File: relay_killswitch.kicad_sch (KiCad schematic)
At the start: 4 parts, among them Q1 BSN20, Q4 Q_PMOS_DGS

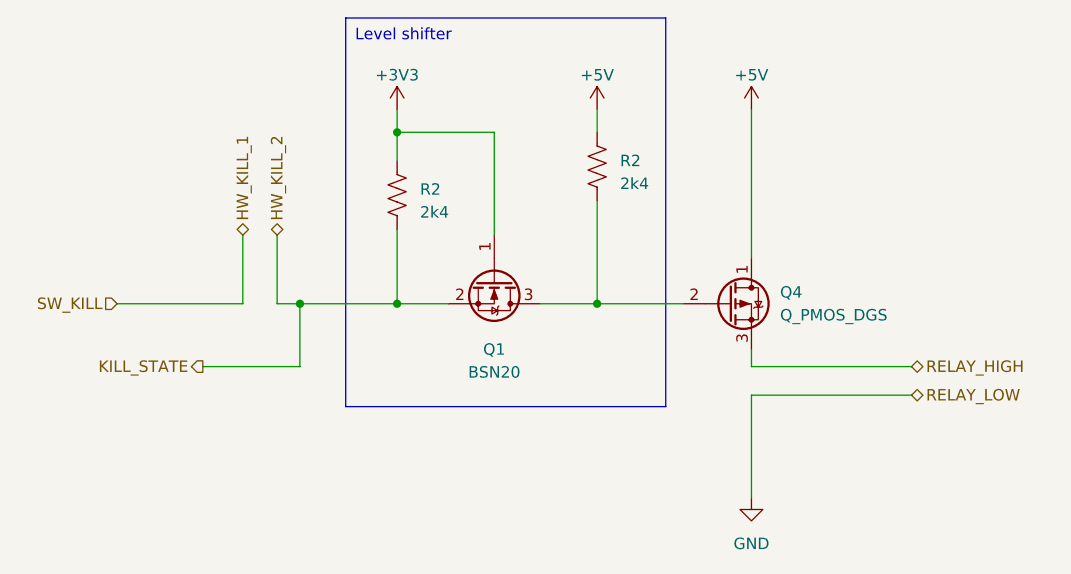
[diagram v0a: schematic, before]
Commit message: Start laying out main board
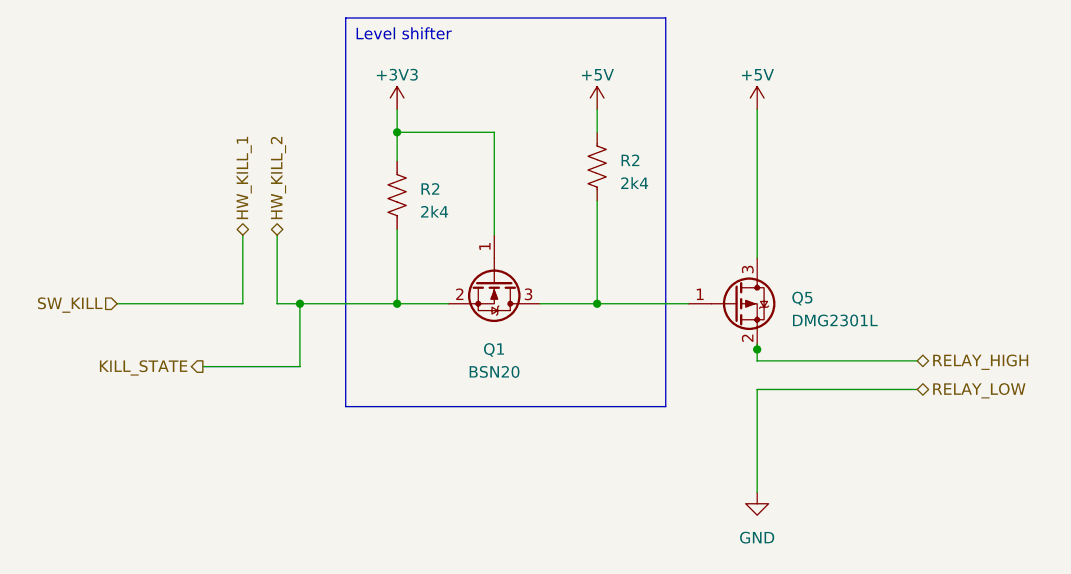
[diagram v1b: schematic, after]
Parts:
- removed Q4: Q_PMOS_DGS, symbol Device:Q_PMOS_DGS
- added Q5: DMG2301L, Package_TO_SOT_SMD:SOT-23, symbol Transistor_FET:DMG2301L
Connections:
- net +5V: now also Q5.3 (D)
- net RELAY_HIGH: now also Q5.2 (S)
- net at Q1.3 (D), R2.2: now also Q5.1 (G)
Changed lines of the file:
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@@
   (junction (at 34.29 49.53) (diameter 0) (color 0 0 0 0)
   )
+  (junction (at 85.09 54.61) (diameter 0) (color 0 0 0 0)
+  )
   (junction (at 45.085 49.53) (diameter 0) (color 0 0 0 0)
   )
@@
   (junction (at 45.085 30.48) (diameter 0) (color 0 0 0 0)
   )
-  (wire (pts (xy 84.455 27.94) (xy 84.455 44.45))
+  (wire (pts (xy 85.09 27.94) (xy 85.09 44.45))
     (stroke (width 0) (type default))
   )
@@
     (stroke (width 0) (type default))
   )
+  (wire (pts (xy 85.09 54.61) (xy 85.09 53.975))
+    (stroke (width 0) (type default))
+  )
   (wire (pts (xy 31.75 49.53) (xy 34.29 49.53))
     (stroke (width 0) (type default))
@@
     (stroke (width 0) (type default))
   )
-  (wire (pts (xy 84.455 56.515) (xy 102.235 56.515))
+  (wire (pts (xy 85.09 55.88) (xy 102.87 55.88))
     (stroke (width 0) (type default))
   )
@@
     (stroke (width 0) (type default))
   )
-  (wire (pts (xy 84.455 59.69) (xy 84.455 71.12))
-    (stroke (width 0) (type default))
-  )
-  (wire (pts (xy 67.31 49.53) (xy 76.835 49.53))
-    (stroke (width 0) (type default))
-  )
-  (wire (pts (xy 84.455 56.515) (xy 84.455 54.61))
-    (stroke (width 0) (type default))
-  )
-  (wire (pts (xy 84.455 59.69) (xy 102.235 59.69))
+  (wire (pts (xy 85.09 59.055) (xy 85.09 70.485))
+    (stroke (width 0) (type default))
+  )
+  (wire (pts (xy 67.31 49.53) (xy 77.47 49.53))
+    (stroke (width 0) (type default))
+  )
+  (wire (pts (xy 85.09 55.88) (xy 85.09 54.61))
+    (stroke (width 0) (type default))
+  )
+  (wire (pts (xy 85.09 59.055) (xy 102.87 59.055))
     (stroke (width 0) (type default))
   )
@@
     (effects (font (size 1.27 1.27)) (justify right))
   )
-  (hierarchical_label "RELAY_HIGH" (shape bidirectional) (at 102.235 56.515 0) (fields_autoplaced)
-    (effects (font (size 1.27 1.27)) (justify left))
-  )
-  (hierarchical_label "RELAY_LOW" (shape bidirectional) (at 102.235 59.69 0) (fields_autoplaced)
-    (effects (font (size 1.27 1.27)) (justify left))
-  )
-  (symbol (lib_id "power:GND") (at 84.455 71.12 0) (unit 1)
-    (in_bom yes) (on_board yes) (dnp no) (fields_autoplaced)
-    (property "Reference" "#PWR051" (at 84.455 77.47 0)
-      (effects (font (size 1.27 1.27)) hide)
-    )
-    (property "Value" "GND" (at 84.455 76.2 0)
-      (effects (font (size 1.27 1.27)))
-    )
-    (property "Footprint" "" (at 84.455 71.12 0)
-      (effects (font (size 1.27 1.27)) hide)
-    )
-    (property "Datasheet" "" (at 84.455 71.12 0)
+  (hierarchical_label "RELAY_HIGH" (shape bidirectional) (at 102.87 55.88 0) (fields_autoplaced)
+    (effects (font (size 1.27 1.27)) (justify left))
+  )
+  (hierarchical_label "RELAY_LOW" (shape bidirectional) (at 102.87 59.055 0) (fields_autoplaced)
+    (effects (font (size 1.27 1.27)) (justify left))
+  )
+  (symbol (lib_id "power:GND") (at 85.09 70.485 0) (unit 1)
+    (in_bom yes) (on_board yes) (dnp no) (fields_autoplaced)
+    (property "Reference" "#PWR051" (at 85.09 76.835 0)
+      (effects (font (size 1.27 1.27)) hide)
+    )
+    (property "Value" "GND" (at 85.09 75.565 0)
+      (effects (font (size 1.27 1.27)))
+    )
+    (property "Footprint" "" (at 85.09 70.485 0)
+      (effects (font (size 1.27 1.27)) hide)
+    )
+    (property "Datasheet" "" (at 85.09 70.485 0)
       (effects (font (size 1.27 1.27)) hide)
     )
@@
         (path "/74b566fe-9d71-4817-95ed-d472d647f8c8/0e721f5c-da80-471e-ad5a-644eccf6c541"
           (reference "#PWR051") (unit 1)
+        )
+      )
+    )
+  )
+  (symbol (lib_id "Transistor_FET:DMG2301L") (at 82.55 49.53 0) (unit 1)
+    (in_bom yes) (on_board yes) (dnp no) (fields_autoplaced)
+    (property "Reference" "Q5" (at 88.9 48.895 0)
+      (effects (font (size 1.27 1.27)) (justify left))
+    )
+    (property "Value" "DMG2301L" (at 88.9 51.435 0)
+      (effects (font (size 1.27 1.27)) (justify left))
+    )
+    (property "Footprint" "Package_TO_SOT_SMD:SOT-23" (at 87.63 51.435 0)
+      (effects (font (size 1.27 1.27) italic) (justify left) hide)
+    )
+    (property "Datasheet" "https://www.diodes.com/assets/Datasheets/DMG2301L.pdf" (at 82.55 49.53 0)
+      (effects (font (size 1.27 1.27)) (justify left) hide)
+    )
+    (pin "1")
+    (pin "2")
+    (pin "3")
+    (instances
+      (project "crush-main-board"
+        (path "/74b566fe-9d71-4817-95ed-d472d647f8c8/0e721f5c-da80-471e-ad5a-644eccf6c541"
+          (reference "Q5") (unit 1)
         )
       )
@@
     )
   )
-  (symbol (lib_id "power:+5V") (at 84.455 27.94 0) (unit 1)
+  (symbol (lib_id "power:+5V") (at 85.09 27.94 0) (unit 1)
     (in_bom yes) (on_board yes) (dnp no)
-    (property "Reference" "#PWR036" (at 84.455 31.75 0)
-      (effects (font (size 1.27 1.27)) hide)
-    )
-    (property "Value" "+5V" (at 84.455 24.13 0)
-      (effects (font (size 1.27 1.27)))
-    )
-    (property "Footprint" "" (at 84.455 27.94 0)
-      (effects (font (size 1.27 1.27)) hide)
-    )
-    (property "Datasheet" "" (at 84.455 27.94 0)
+    (property "Reference" "#PWR036" (at 85.09 31.75 0)
+      (effects (font (size 1.27 1.27)) hide)
+    )
+    (property "Value" "+5V" (at 85.09 24.13 0)
+      (effects (font (size 1.27 1.27)))
+    )
+    (property "Footprint" "" (at 85.09 27.94 0)
+      (effects (font (size 1.27 1.27)) hide)
+    )
+    (property "Datasheet" "" (at 85.09 27.94 0)
       (effects (font (size 1.27 1.27)) hide)
     )
@@
         )
       )
-    )
-  )
-  (symbol (lib_id "Device:Q_PMOS_DGS") (at 81.915 49.53 0) (unit 1)
-    (in_bom yes) (on_board yes) (dnp no) (fields_autoplaced)
-    (property "Reference" "Q4" (at 87.63 48.26 0)
-      (effects (font (size 1.27 1.27)) (justify left))
-    )
-    (property "Value" "Q_PMOS_DGS" (at 87.63 50.8 0)
-      (effects (font (size 1.27 1.27)) (justify left))
-    )
-    (property "Footprint" "" (at 86.995 46.99 0)
-      (effects (font (size 1.27 1.27)) hide)
-    )
-    (property "Datasheet" "~" (at 81.915 49.53 0)
-      (effects (font (size 1.27 1.27)) hide)
-    )
-    (pin "1")
-    (pin "2")
-    (pin "3")
-    (instances
-      (project "crush-main-board"
-        (path "/74b566fe-9d71-4817-95ed-d472d647f8c8/0e721f5c-da80-471e-ad5a-644eccf6c541"
-          (reference "Q4") (unit 1)
-        )
-      )
